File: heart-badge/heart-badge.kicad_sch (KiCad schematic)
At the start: 18 parts, among them SW1 SW_SPDT

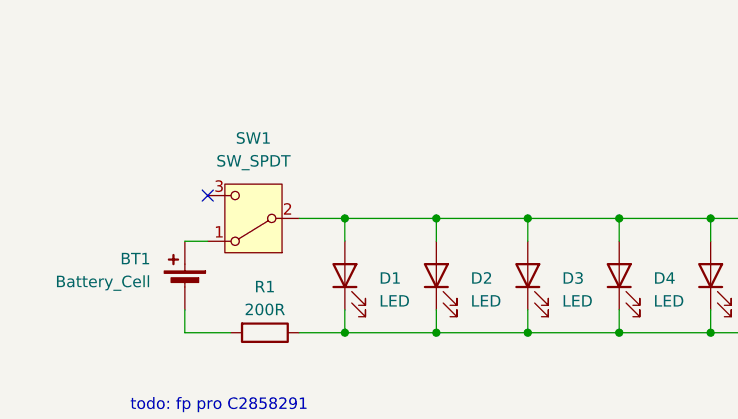
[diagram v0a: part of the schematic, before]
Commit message: heart-badge development
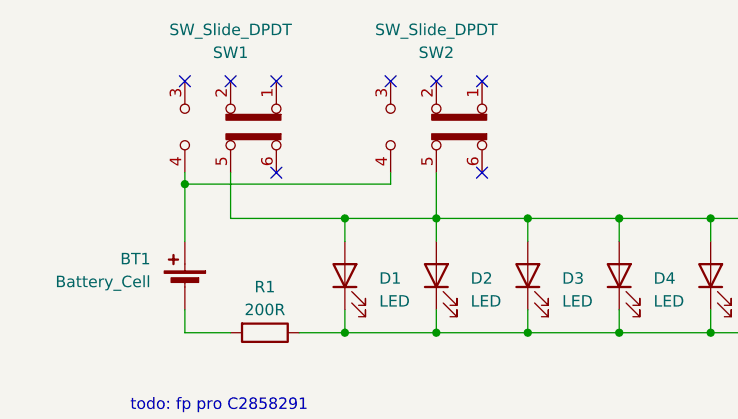
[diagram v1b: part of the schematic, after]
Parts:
- removed SW1: SW_SPDT, symbol Switch:SW_SPDT
- added SW1, SW2: SW_Slide_DPDT, symbol Switch:SW_Slide_DPDT
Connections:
- net at D1.2 (A), D10.2 (A), D11.2 (A)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: now also SW1.5 (B), SW2.5 (B)
- net at BT1.1 (+): now also SW1.4 (A), SW2.4 (A)
- no-connect marks 1 -> 8
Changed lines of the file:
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@@
+	)
+	(junction
+		(at 109.22 69.85)
+		(diameter 0)
+		(color 0 0 0 0)
 	)
 	(junction
@@
 	)
 	(no_connect
-		(at 111.76 71.12)
+		(at 132.08 58.42)
+	)
+	(no_connect
+		(at 142.24 68.58)
+	)
+	(no_connect
+		(at 142.24 58.42)
+	)
+	(no_connect
+		(at 109.22 58.42)
+	)
+	(no_connect
+		(at 119.38 58.42)
+	)
+	(no_connect
+		(at 114.3 58.42)
+	)
+	(no_connect
+		(at 137.16 58.42)
+	)
+	(no_connect
+		(at 119.38 68.58)
 	)
 	(wire
@@
 	(wire
 		(pts
-			(xy 121.92 73.66) (xy 127 73.66)
-		)
-		(stroke
-			(width 0)
-			(type default)
-		)
-	)
-	(wire
-		(pts
 			(xy 259.08 73.66) (xy 259.08 76.2)
 		)
@@
 	(wire
 		(pts
-			(xy 109.22 76.2) (xy 111.76 76.2)
+			(xy 114.3 73.66) (xy 127 73.66)
 		)
 		(stroke
@@
 	(wire
 		(pts
+			(xy 109.22 68.58) (xy 109.22 69.85)
+		)
+		(stroke
+			(width 0)
+			(type default)
+		)
+	)
+	(wire
+		(pts
 			(xy 228.6 73.66) (xy 238.76 73.66)
 		)
@@
 	(wire
 		(pts
+			(xy 132.08 69.85) (xy 132.08 68.58)
+		)
+		(stroke
+			(width 0)
+			(type default)
+		)
+	)
+	(wire
+		(pts
 			(xy 269.24 73.66) (xy 269.24 76.2)
 		)
@@
 	(wire
 		(pts
+			(xy 109.22 69.85) (xy 109.22 76.2)
+		)
+		(stroke
+			(width 0)
+			(type default)
+		)
+	)
+	(wire
+		(pts
 			(xy 259.08 86.36) (xy 259.08 83.82)
 		)
@@
 	(wire
 		(pts
+			(xy 109.22 69.85) (xy 132.08 69.85)
+		)
+		(stroke
+			(width 0)
+			(type default)
+		)
+	)
+	(wire
+		(pts
 			(xy 109.22 86.36) (xy 114.3 86.36)
 		)
@@
 	(wire
 		(pts
+			(xy 114.3 68.58) (xy 114.3 73.66)
+		)
+		(stroke
+			(width 0)
+			(type default)
+		)
+	)
+	(wire
+		(pts
 			(xy 167.64 86.36) (xy 177.8 86.36)
 		)
@@
 		(pts
 			(xy 177.8 73.66) (xy 177.8 76.2)
+		)
+		(stroke
+			(width 0)
+			(type default)
+		)
+	)
+	(wire
+		(pts
+			(xy 137.16 68.58) (xy 137.16 73.66)
 		)
 		(stroke
@@
 	)
 	(symbol
-		(lib_id "Switch:SW_SPDT")
-		(at 116.84 73.66 180)
-		(unit 1)
-		(exclude_from_sim no)
-		(in_bom yes)
-		(on_board yes)
-		(dnp no)
-		(fields_autoplaced yes)
-		(property "Reference" "SW1"
-			(at 116.84 64.77 0)
-			(effects
-				(font
-					(size 1.27 1.27)
-				)
-			)
-		)
-		(property "Value" "SW_SPDT"
-			(at 116.84 67.31 0)
-			(effects
-				(font
-					(size 1.27 1.27)
-				)
-			)
-		)
-		(property "Footprint" ""
-			(at 116.84 73.66 0)
-			(effects
-				(font
-					(size 1.27 1.27)
-				)
-				(hide yes)
-			)
-		)
-		(property "Datasheet" "~"
-			(at 116.84 66.04 0)
-			(effects
-				(font
-					(size 1.27 1.27)
-				)
-				(hide yes)
-			)
-		)
-		(property "Description" "Switch, single pole double throw"
-			(at 116.84 73.66 0)
-			(effects
-				(font
-					(size 1.27 1.27)
-				)
-				(hide yes)
-			)
-		)
-		(pin "1"
-		)
-		(pin "3"
-		)
-		(pin "2"
-		)
-		(instances
-			(project "heart-badge"
-				(path "/e40cfca1-d107-4c96-90fb-8f9c14af6cf6"
-					(reference "SW1")
-					(unit 1)
-				)
-			)
-		)
-	)
-	(symbol
 		(lib_id "Device:LED")
 		(at 259.08 80.01 90)
@@
 					(unit 1)
 				)
+			)
+		)
+	)
+	(symbol
+		(lib_id "Switch:SW_Slide_DPDT")
+		(at 137.16 63.5 270)
+		(unit 1)
+		(exclude_from_sim no)
+		(in_bom yes)
+		(on_board yes)
+		(dnp no)
+		(property "Reference" "SW2"
+			(at 137.16 55.245 90)
+			(effects
+				(font
+					(size 1.27 1.27)
+				)
+			)
+		)
+		(property "Value" "SW_Slide_DPDT"
+			(at 137.16 52.705 90)
+			(effects
+				(font
+					(size 1.27 1.27)
+				)
+			)
+		)
+		(property "Footprint" ""
+			(at 142.24 77.47 0)
+			(effects
+				(font
+					(size 1.27 1.27)
+				)
+				(hide yes)
+			)
+		)
+		(property "Datasheet" "~"
+			(at 137.16 63.5 0)
+			(effects
+				(font
+					(size 1.27 1.27)
+				)
+				(hide yes)
+			)
+		)
+		(property "Description" "Slide Switch, dual pole double throw"
+			(at 137.16 63.5 0)
+			(effects
+				(font
+					(size 1.27 1.27)
+				)
+				(hide yes)
+			)
+		)
+		(pin "3"
+		)
+		(pin "4"
+		)
+		(pin "5"
+		)
+		(pin "6"
+		)
+		(pin "1"
+		)
+		(pin "2"
+		)
+		(instances
+			(project "heart-badge"
+				(path "/e40cfca1-d107-4c96-90fb-8f9c14af6cf6"
+					(reference "SW2")
+					(unit 1)
+				)
+			)
+		)
+	)
+	(symbol
+		(lib_id "Switch:SW_Slide_DPDT")
+		(at 114.3 63.5 270)
+		(unit 1)
+		(exclude_from_sim no)
+		(in_bom yes)
+		(on_board yes)
+		(dnp no)
+		(property "Reference" "SW1"
+			(at 114.3 55.245 90)
+			(effects
+				(font
+					(size 1.27 1.27)
+				)
+			)
+		)
+		(property "Value" "SW_Slide_DPDT"
+			(at 114.3 52.705 90)
+			(effects
+				(font
+					(size 1.27 1.27)
+				)
+			)
+		)
+		(property "Footprint" ""
+			(at 119.38 77.47 0)
+			(effects
+				(font
+					(size 1.27 1.27)
+				)
+				(hide yes)
+			)
+		)
+		(property "Datasheet" "~"
+			(at 114.3 63.5 0)
+			(effects
+				(font
+					(size 1.27 1.27)
+				)
+				(hide yes)
+			)
+		)
+		(property "Description" "Slide Switch, dual pole double throw"
+			(at 114.3 63.5 0)
+			(effects
+				(font
+					(size 1.27 1.27)
+				)
+				(hide yes)
+			)
+		)
+		(pin "3"
+		)
+		(pin "4"
+		)
+		(pin "5"
+		)
+		(pin "6"
+		)
+		(pin "1"
+		)
+		(pin "2"
+		)
+		(instances
+			(project "heart-badge"
+				(path "/e40cfca1-d107-4c96-90fb-8f9c14af6cf6"
+					(reference "SW1")
+					(unit 1)
+				)
